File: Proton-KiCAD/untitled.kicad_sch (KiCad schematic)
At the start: 41 parts, among them J2 KEYPAD, J3 AudioJack3, J4 SPEAKER_OUT, J5 OLED SPI, J6 ROTARY ENCODER, J7 OLED, J8 SI4703, U5 TL072, U6 LM386

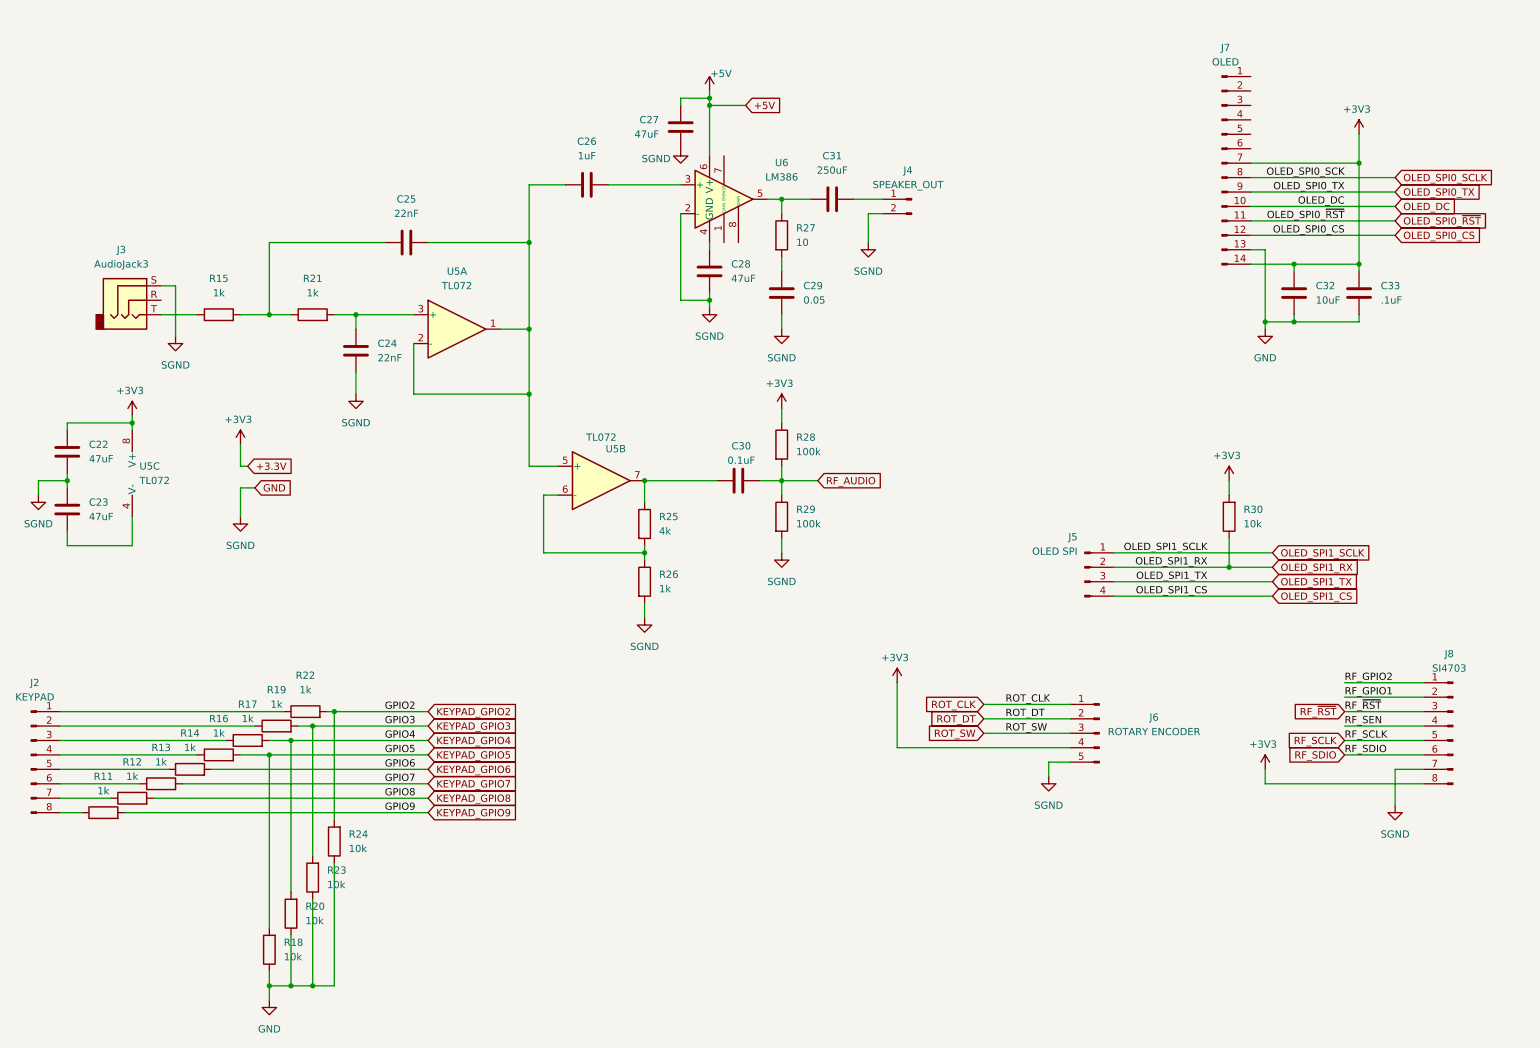
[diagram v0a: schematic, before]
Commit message: ready for final check
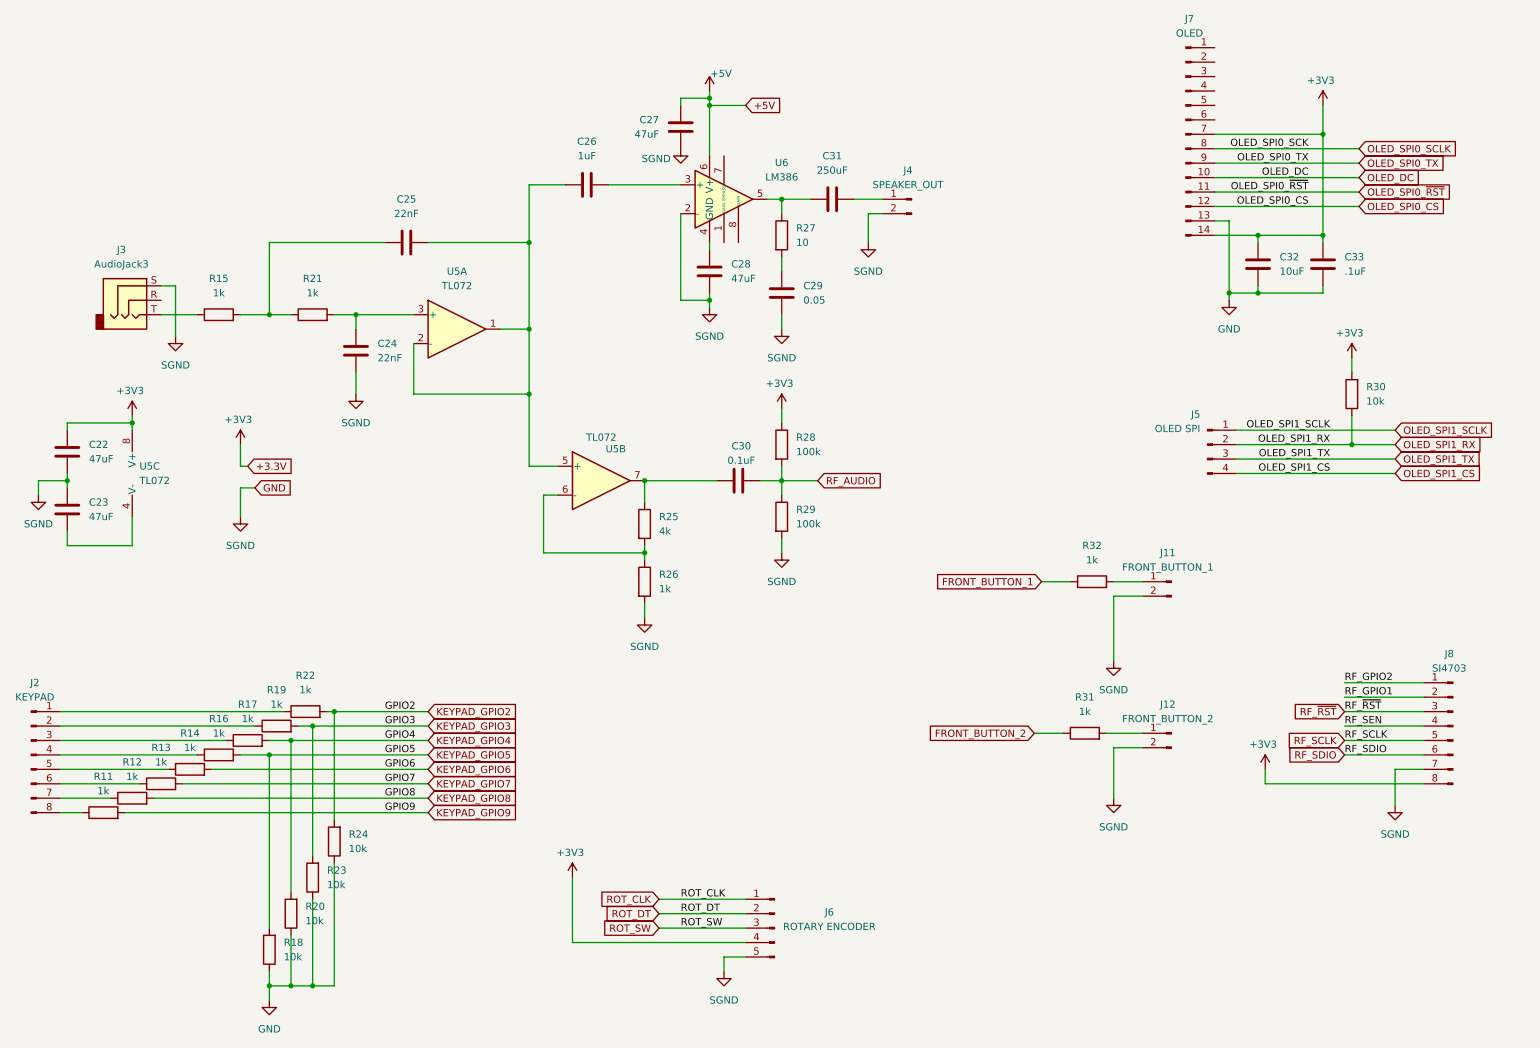
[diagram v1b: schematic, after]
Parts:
- added J11: FRONT_BUTTON_1, Connector_PinHeader_2.54mm:PinHeader_1x02_P2.54mm_Vertical, symbol Connector:Conn_01x02_Pin
- added J12: FRONT_BUTTON_2, Connector_PinHeader_2.54mm:PinHeader_1x02_P2.54mm_Vertical, symbol Connector:Conn_01x02_Pin
- added R31, R32: 1k, Resistor_SMD:R_0402_1005Metric, symbol Device:R
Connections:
- net GND: now also J11.2 (Pin_2), J12.2 (Pin_2)
- new net: J12.1 (Pin_1), R31.2
- new net: J11.1 (Pin_1), R32.2
- new net FRONT_BUTTON_1: R32.1
- new net FRONT_BUTTON_2: R31.1
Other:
- moved on the sheet: C32, C33, J5, J6, J7, R30
